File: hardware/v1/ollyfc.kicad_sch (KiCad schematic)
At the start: 64 parts, among them J1 Conn_01x06, J5 Conn_02x05_Odd_Even, Q2 MMBT3904, Q3 MMBT3904, SW2 SW_Push, SW4 MODE1, SW5 MODE1, U3 STM32F411RETx, U6 W25Q128JVS, Y1 X322516MLB4SI

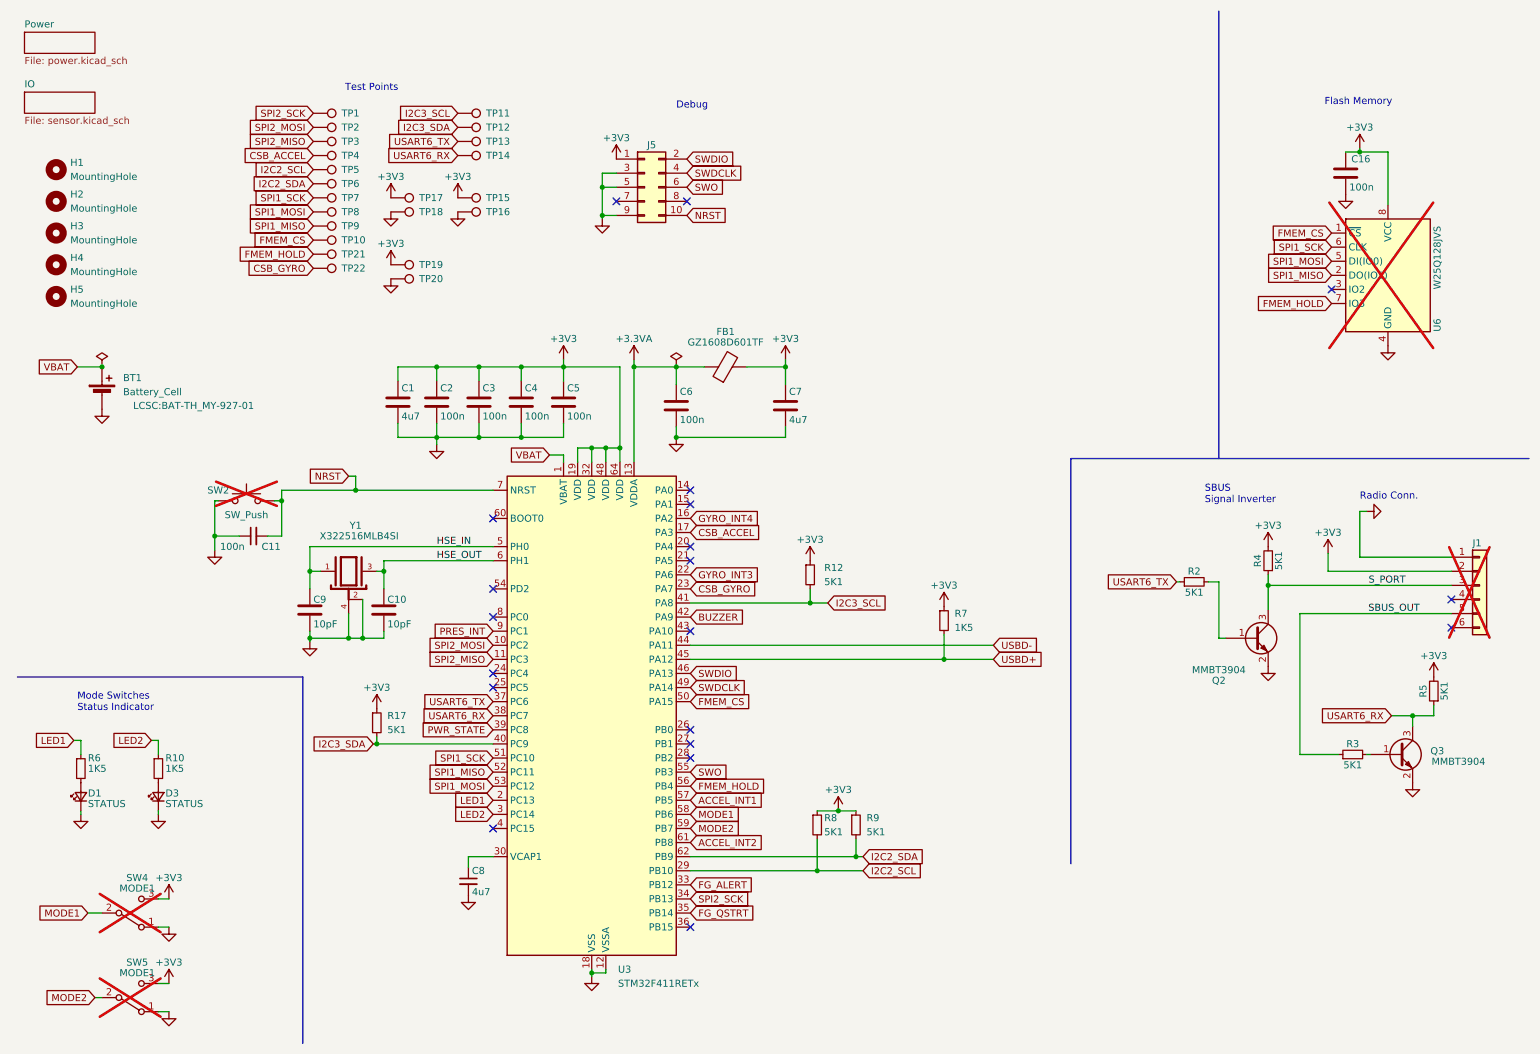
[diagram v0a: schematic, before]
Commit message: some hardware designs
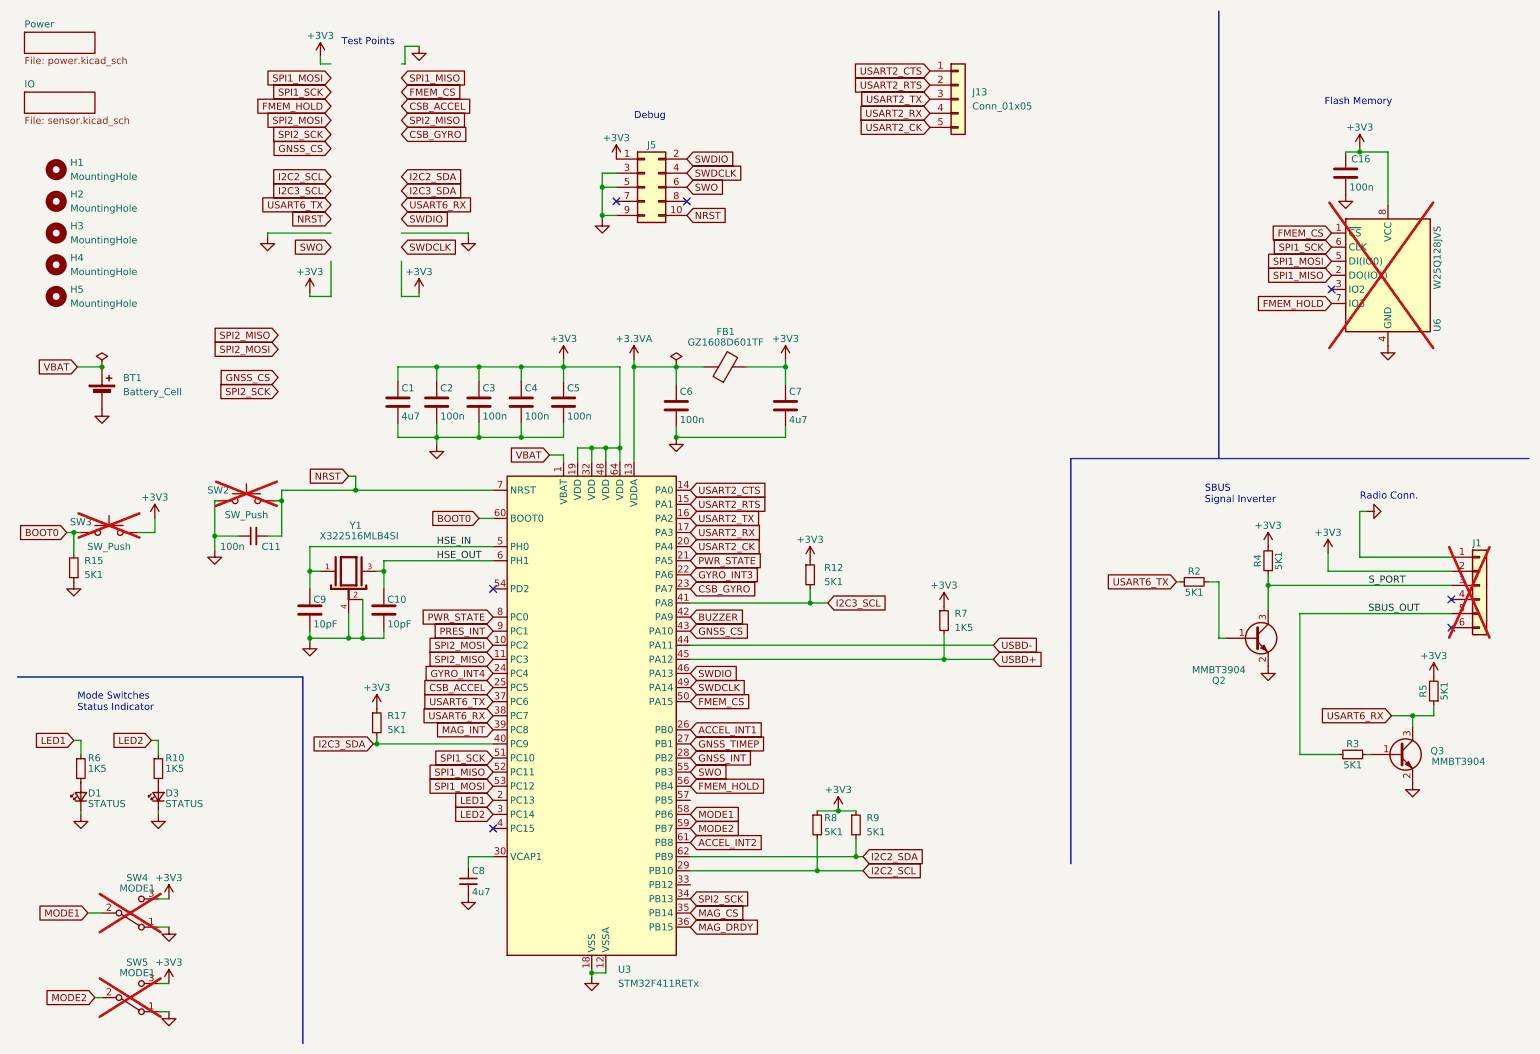
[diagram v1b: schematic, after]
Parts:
- removed TP1, TP10, TP11, TP12, TP13, TP14, TP15, TP16, TP17, TP18, TP19, TP2, TP20, TP21, TP22, TP3, TP4, TP5, TP6, TP7, TP8, TP9: TestPoint, TestPoint:TestPoint_THTPad_D1.0mm_Drill0.5mm, symbol Connector:TestPoint
- added J13: Conn_01x05, Connector_PinHeader_2.54mm:PinHeader_1x05_P2.54mm_Vertical, symbol Connector_Generic:Conn_01x05
- added R15: 5K1, Resistor_SMD:R_0402_1005Metric, symbol Device:R_Small
- added SW3: SW_Push, Button_Switch_THT:SW_PUSH_6mm, symbol Switch:SW_Push
- BT1: footprint LCSC:BAT-TH_MY-927-01 -> Battery:BatteryHolder_Keystone_3002_1x2032
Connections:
- net +3V3: now also SW3.2
- net ACCEL_INT1: now also U3.26 (PB0); no longer U3.57 (PB5)
- net CSB_ACCEL: now also U3.25 (PC5); no longer U3.17 (PA3)
- net GND: now also R15.1
- net GYRO_INT4: now also U3.24 (PC4); no longer U3.16 (PA2)
- net PWR_STATE: now also U3.21 (PA5), U3.8 (PC0); no longer U3.39 (PC8)
- net USART2_CTS: now reaches U3.14 (PA0)
- net USART2_CTS: now also J13.1 (Pin_1)
- net USART2_RTS: now reaches U3.15 (PA1)
- net USART2_RTS: now also J13.2 (Pin_2)
- net USART2_CK: now reaches U3.20 (PA4)
- net USART2_CK: now also J13.5 (Pin_5)
- net GNSS_TIMEP: now reaches U3.27 (PB1)
- net GNSS_INT: now reaches U3.28 (PB2)
- net MAG_DRDY: now reaches U3.36 (PB15)
- net GNSS_CS: now reaches U3.43 (PA10)
- net BOOT0: now reaches U3.60 (BOOT0)
- net BOOT0: now also R15.2, SW3.1
- net FG_ALERT: no longer names the net of U3.33 (PB12)
- net FG_QSTRT renamed MAG_CS
- new net MAG_INT: U3.39 (PC8)
- new net USART2_RX: J13.4 (Pin_4), U3.17 (PA3)
- new net USART2_TX: J13.3 (Pin_3), U3.16 (PA2)
- no-connect marks 20 -> 7

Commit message: Route another?
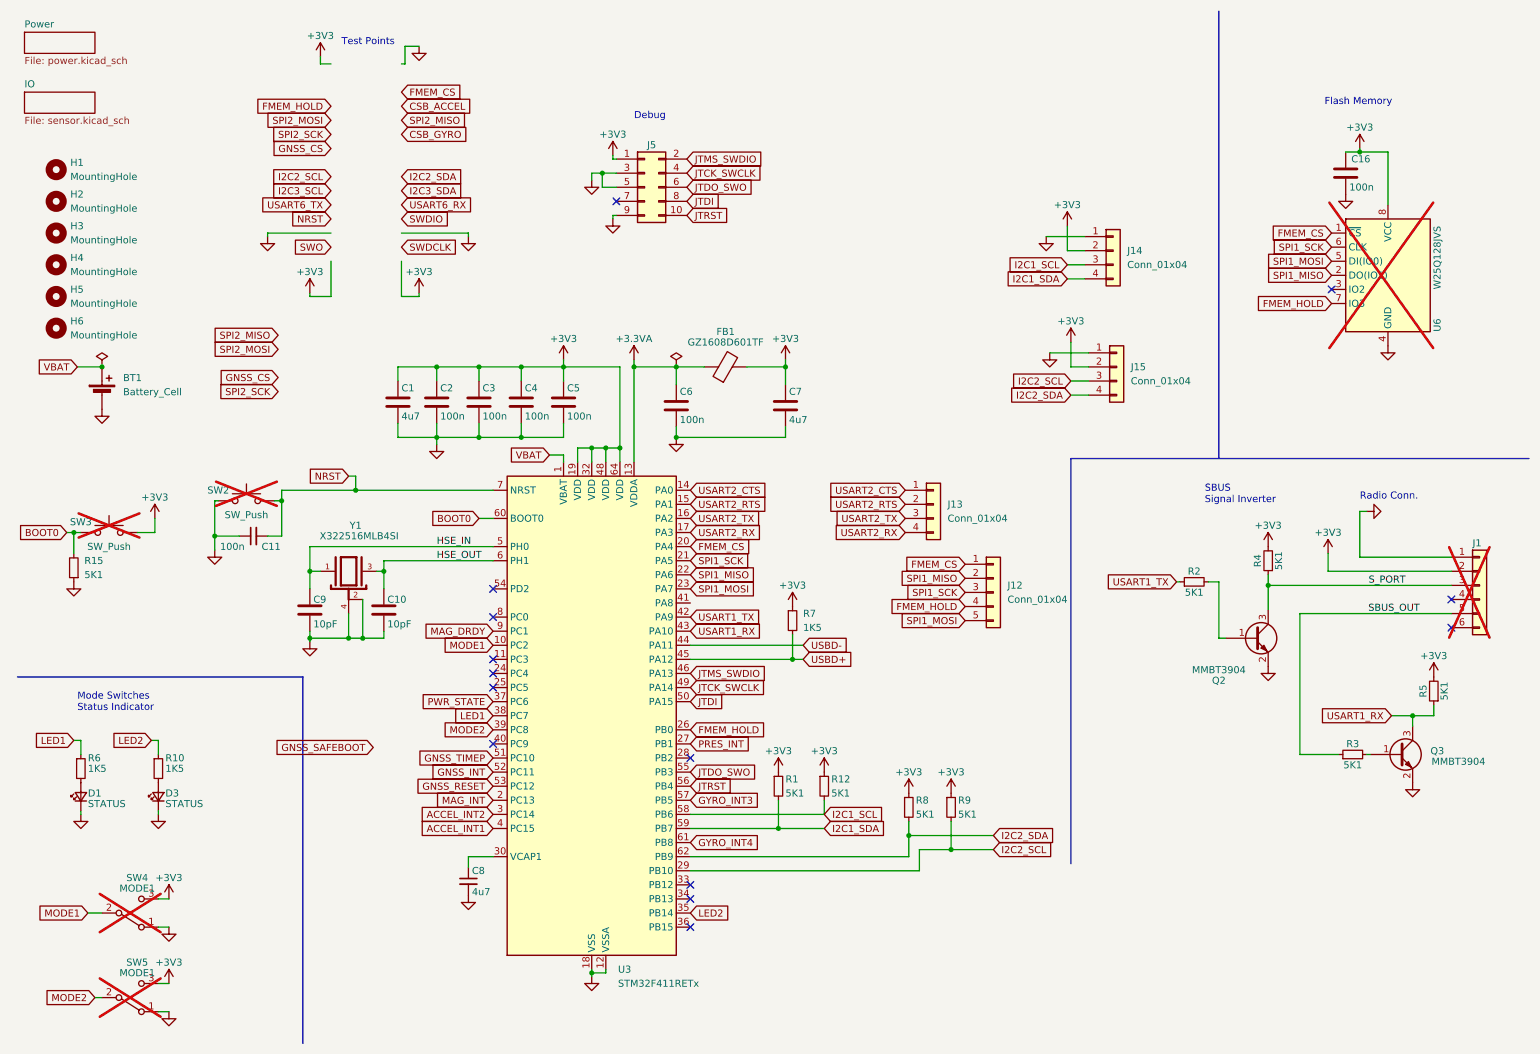
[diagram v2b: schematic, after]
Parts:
- removed R17: 5K1, Resistor_SMD:R_0402_1005Metric, symbol Device:R_Small
- added H6: MountingHole, MountingHole:MountingHole_3.2mm_M3, symbol Mechanical:MountingHole
- added J12: Conn_01x04, Connector_PinHeader_2.54mm:PinHeader_1x05_P2.54mm_Vertical, symbol Connector_Generic:Conn_01x05
- added J14, J15: Conn_01x04, Connector_PinHeader_2.54mm:PinHeader_1x04_P2.54mm_Vertical, symbol Connector_Generic:Conn_01x04
- added R1: 5K1, Resistor_SMD:R_0402_1005Metric, symbol Device:R_Small
- J13: value Conn_01x05 -> Conn_01x04; footprint Connector_PinHeader_2.54mm:PinHeader_1x05_P2.54mm_Vertical -> Connector_PinHeader_2.54mm:PinHeader_1x04_P2.54mm_Vertical; symbol Connector_Generic:Conn_01x05 -> Connector_Generic:Conn_01x04
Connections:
- net MAG_CS is gone; now on net LED2: U3.35 (PB14)
- net +3V3: now also J14.2 (Pin_2), J15.2 (Pin_2), R1.1
- net ACCEL_INT1: now also U3.4 (PC15); no longer U3.26 (PB0)
- net ACCEL_INT2: now also U3.3 (PC14); no longer U3.61 (PB8)
- net CSB_ACCEL: no longer U3.25 (PC5)
- net CSB_GYRO: no longer U3.23 (PA7)
- net FMEM_CS: now also U3.20 (PA4), J12.1 (Pin_1); no longer U3.50 (PA15)
- net FMEM_HOLD: now also U3.26 (PB0), J12.4 (Pin_4); no longer U3.56 (PB4)
- net GND: now also J14.1 (Pin_1), J15.1 (Pin_1)
- net GNSS_CS: no longer U3.43 (PA10)
- net GNSS_INT: now also U3.52 (PC11); no longer U3.28 (PB2)
- net GNSS_TIMEP: now also U3.51 (PC10); no longer U3.27 (PB1)
- net GYRO_INT3: now also U3.57 (PB5); no longer U3.22 (PA6)
- net GYRO_INT4: now also U3.61 (PB8); no longer U3.24 (PC4)
- net I2C2_SCL: now also R9.2, J15.3 (Pin_3); no longer R8.2
- net I2C2_SDA: now also R8.2, J15.4 (Pin_4); no longer R9.2
- net I2C3_SCL: no longer R12.2, U3.41 (PA8)
- net I2C3_SDA: no longer U3.40 (PC9)
- net LED1: now also U3.38 (PC7); no longer U3.2 (PC13)
- net LED2: no longer U3.3 (PC14)
- net MAG_DRDY: now also U3.9 (PC1); no longer U3.36 (PB15)
- net MAG_INT: now also U3.2 (PC13); no longer U3.39 (PC8)
- net MODE1: now also U3.10 (PC2); no longer U3.58 (PB6)
- net MODE2: now also U3.39 (PC8); no longer U3.59 (PB7)
- net NRST: no longer J5.10 (Pin_10)
- net PRES_INT: now also U3.27 (PB1); no longer U3.9 (PC1)
- net PWR_STATE: now also U3.37 (PC6); no longer U3.21 (PA5), U3.8 (PC0)
- net SPI1_MISO: now also U3.22 (PA6), J12.2 (Pin_2); no longer U3.52 (PC11)
- net SPI1_MOSI: now also U3.23 (PA7), J12.5 (Pin_5); no longer U3.53 (PC12)
- net SPI1_SCK: now also U3.21 (PA5), J12.3 (Pin_3); no longer U3.51 (PC10)
- net SPI2_MISO: no longer U3.11 (PC3)
- net SPI2_MOSI: no longer U3.10 (PC2)
- net SPI2_SCK: no longer U3.34 (PB13)
- net SWDCLK: no longer J5.4 (Pin_4), U3.49 (PA14)
- net SWDIO: no longer J5.2 (Pin_2), U3.46 (PA13)
- net SWO: no longer J5.6 (Pin_6), U3.55 (PB3)
- net USART6_RX: no longer Q3.3 (C), R5.1, U3.38 (PC7)
- net USART6_TX: no longer R2.1, U3.37 (PC6)
- net JTDI: now reaches J5.8 (Pin_8)
- net JTDI: now also U3.50 (PA15)
- net BUZZER renamed USART1_TX
- net USART1_TX: now also R2.1
- removed net USART2_CK: J13.5 (Pin_5), U3.20 (PA4)
- new net GNSS_RESET: U3.53 (PC12)
- new net I2C1_SCL: J14.3 (Pin_3), R12.2, U3.58 (PB6)
- new net I2C1_SDA: J14.4 (Pin_4), R1.2, U3.59 (PB7)
- new net JTCK_SWCLK: J5.4 (Pin_4), U3.49 (PA14)
- new net JTDO_SWO: J5.6 (Pin_6), U3.55 (PB3)
- new net JTMS_SWDIO: J5.2 (Pin_2), U3.46 (PA13)
- new net JTRST: J5.10 (Pin_10), U3.56 (PB4)
- new net USART1_RX: Q3.3 (C), R5.1, U3.43 (PA10)
- no-connect marks 7 -> 14
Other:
- moved on the sheet: R12, R7
